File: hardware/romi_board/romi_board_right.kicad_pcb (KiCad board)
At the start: 2 copper layers, 99.1 x 66 mm, 33 parts, among them J1 Conn_01x14, J2 Conn_01x14, J3 Conn_01x04, SW1 SW_SPST, U1 Teensy4.0

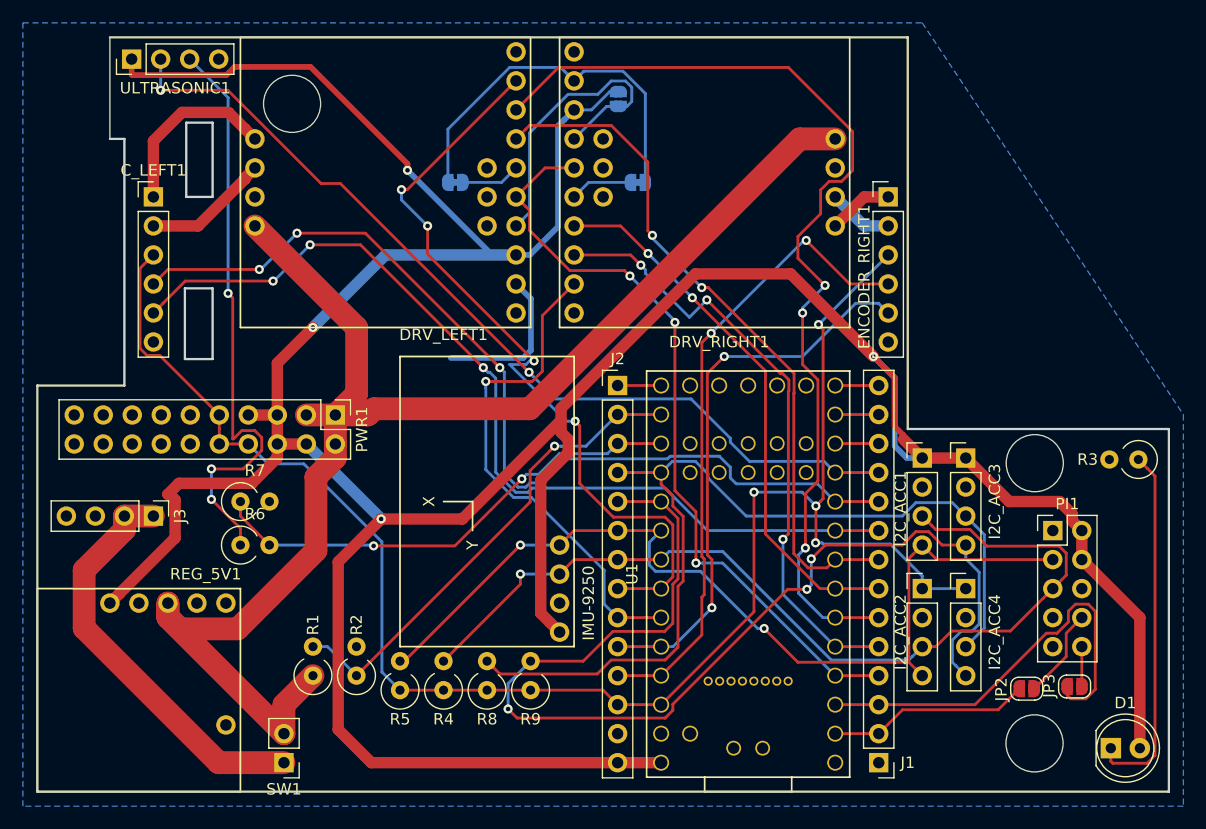
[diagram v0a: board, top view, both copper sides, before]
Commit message: Initial version of schematics and boards.
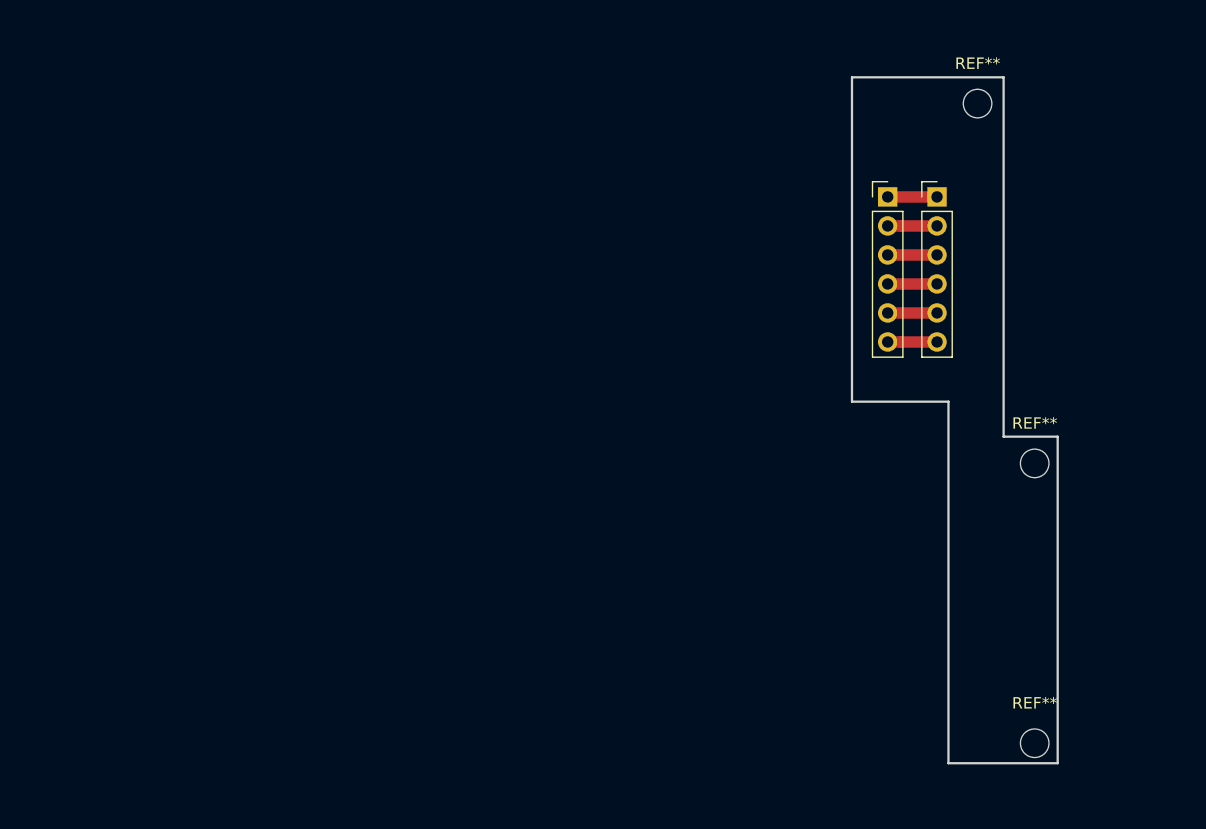
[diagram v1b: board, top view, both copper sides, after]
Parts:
- removed C_LEFT1: Conn_01x07, Connector_PinHeader_2.54mm:PinHeader_1x06_P2.54mm_Vertical
- removed D1: LED, LED_THT:LED_D5.0mm
- removed DRV_LEFT1, DRV_RIGHT1: TB9051FTG, teensy:TB9051FTG_db
- removed I2C_ACC1, I2C_ACC2, I2C_ACC3, I2C_ACC4, J3, ULTRASONIC1: Conn_01x04, Connector_PinHeader_2.54mm:PinHeader_1x04_P2.54mm_Vertical
- removed IMU-9250: Conn_01x04, teensy:MPU9250_BB
- removed J1, J2: Conn_01x14, Connector_PinHeader_2.54mm:PinHeader_1x14_P2.54mm_Vertical
- removed JP1, JP2, JP3: SolderJumper_2_Open, Jumper:SolderJumper-2_P1.3mm_Open_RoundedPad1.0x1.5mm
- removed JP4, JP5: SolderJumper_2_Bridged, Jumper:SolderJumper-2_P1.3mm_Bridged_RoundedPad1.0x1.5mm
- removed PI1: RASPBERRY_PI_GPIO, Connector_PinHeader_2.54mm:PinHeader_2x05_P2.54mm_Vertical
- removed PWR1: Conn_02x10_Counter_Clockwise, Connector_PinHeader_2.54mm:PinHeader_2x10_P2.54mm_Vertical
- removed R1, R2, R3, R4, R5, R8, R9: R_US, Resistor_THT:R_Axial_DIN0309_L9.0mm_D3.2mm_P2.54mm_Vertical
- removed R6, R7: R_Small_US, Resistor_THT:R_Axial_DIN0309_L9.0mm_D3.2mm_P2.54mm_Vertical
- removed REG_5V1: D24V22F5, teensy:D24V2F5_bb
- removed SW1: SW_SPST, Connector_PinHeader_2.54mm:PinHeader_1x02_P2.54mm_Vertical
- removed U1: Teensy4.0, teensy:Teensy40_SMT
- added C_RIGHTx1: Conn_01x07, Connector_PinHeader_2.54mm:PinHeader_1x06_P2.54mm_Vertical, F.Cu at (133.5, 101.3)
- added REF**: MountingHole_2.5mm, MountingHole:MountingHole_2.5mm, F.Cu at (146.3, 149.1)
- added REF**: MountingHole_2.5mm, MountingHole:MountingHole_2.5mm, F.Cu at (146.3, 124.6)
- added REF**: MountingHole_2.5mm, MountingHole:MountingHole_2.5mm, F.Cu at (141.3, 93.1)
- moved ENCODER_RIGHT1 4.27 mm to (137.8, 101.3)
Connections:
- ENCODER_RIGHT1 pad 1: /RM1 -> /RM1x
- ENCODER_RIGHT1 pad 2: /RM2 -> /RM2x
- ENCODER_RIGHT1 pad 3: +3V3 -> /R5V
- ENCODER_RIGHT1 pad 4: /RENCA -> /RENCAx
- ENCODER_RIGHT1 pad 5: /RENCB -> /RENCBx
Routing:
- net +5V: track 318.9 -> 0.00 mm, vias 4 -> 0
- net +3V3: track 146.9 -> 0.00 mm, vias 4 -> 0
- net +VSW: track 129.1 -> 0.00 mm
- net /I2C2_SDA: track 97.3 -> 0.00 mm, vias 3 -> 0
- net /LD_PWM1: track 87.3 -> 0.00 mm, vias 3 -> 0
- net /LENCA: track 83.1 -> 0.00 mm, vias 3 -> 0
- net /I2C1_SCL: track 81.9 -> 0.00 mm, vias 1 -> 0
- net /I2C1_SDA: track 81.6 -> 0.00 mm, vias 2 -> 0
- net /LENCB: track 81.5 -> 0.00 mm, vias 3 -> 0
- net /I2C2_SCL: track 81.2 -> 0.00 mm
- net /US_TRIG: track 79.7 -> 0.00 mm, vias 2 -> 0
- net /LD_OCM: track 68.9 -> 0.00 mm, vias 4 -> 0
- net /XD_EN: track 67.6 -> 0.00 mm, vias 3 -> 0
- net /LD_PWM2: track 61.5 -> 0.00 mm, vias 2 -> 0
- net /RENCA: track 55.9 -> 0.00 mm, vias 2 -> 0
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- removed copper zone on B.Cu, net GND
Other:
- board size 99.1 x 66 mm -> 18 x 60 mm
- net class Motor removed
- net class Supply removed
